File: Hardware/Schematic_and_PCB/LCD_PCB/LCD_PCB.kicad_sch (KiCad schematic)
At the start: 10 parts, among them J1 LCD_display, J2 Conn_01x10, SW1 Button_down, SW2 Button_up, SW3 Button_ok, SW4 Button_back, SW5 SW_Push

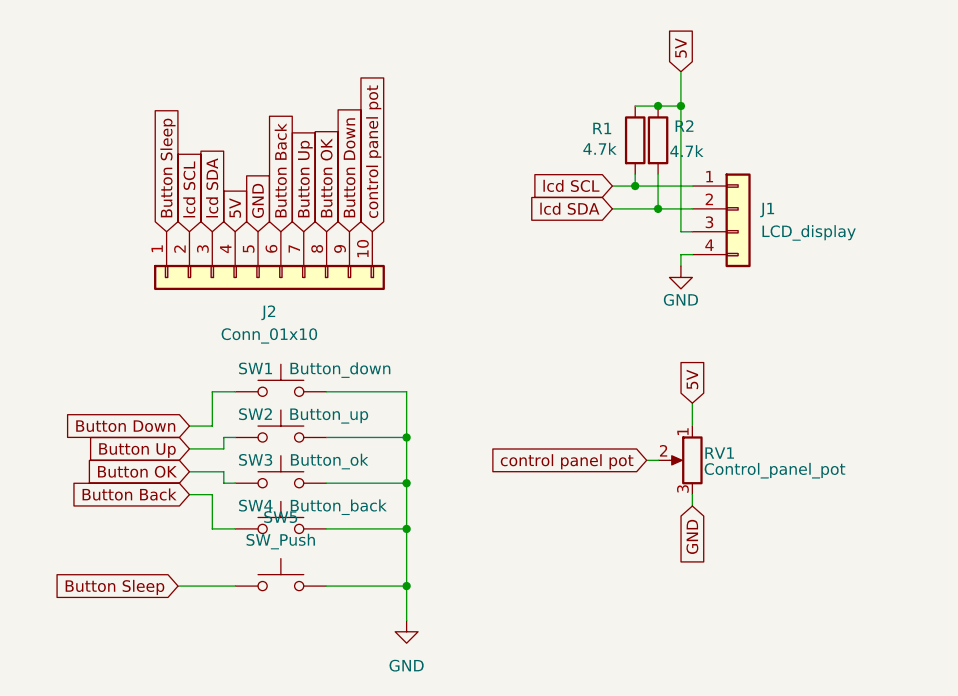
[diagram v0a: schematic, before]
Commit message: Update bunch of stuff
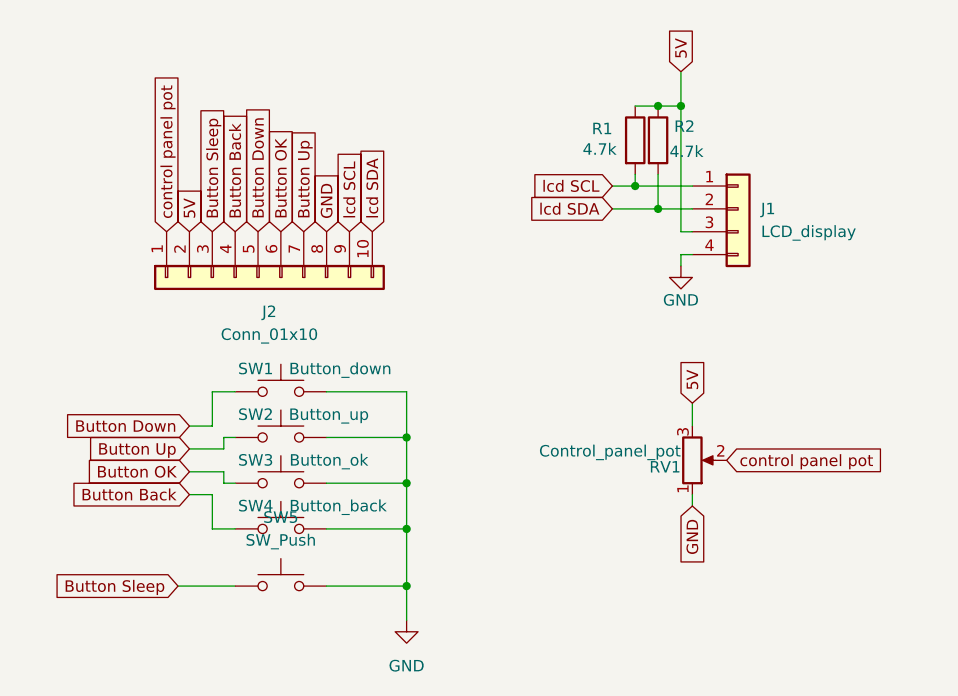
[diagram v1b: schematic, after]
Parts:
- RV1: footprint Potentiometer:PDB182-K-Potentiometer -> Potentiometer:PDB182-K-Potentiometer-Horizontal
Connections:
- net 5V: now also J2.2 (Pin_2), RV1.3; no longer J2.4 (Pin_4), RV1.1
- net Button Back: now also J2.4 (Pin_4); no longer J2.6 (Pin_6)
- net Button Down: now also J2.5 (Pin_5); no longer J2.9 (Pin_9)
- net Button OK: now also J2.6 (Pin_6); no longer J2.8 (Pin_8)
- net Button Sleep: now also J2.3 (Pin_3); no longer J2.1 (Pin_1)
- net GND: now also J2.8 (Pin_8), RV1.1; no longer J2.5 (Pin_5), RV1.3
- net control panel pot: now also J2.1 (Pin_1); no longer J2.10 (Pin_10)
- net lcd SCL: now also J2.9 (Pin_9); no longer J2.2 (Pin_2)
- net lcd SDA: now also J2.10 (Pin_10); no longer J2.3 (Pin_3)
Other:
- moved on the sheet: RV1
